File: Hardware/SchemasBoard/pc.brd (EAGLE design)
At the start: 14.9 x 24.1 mm, 10 parts

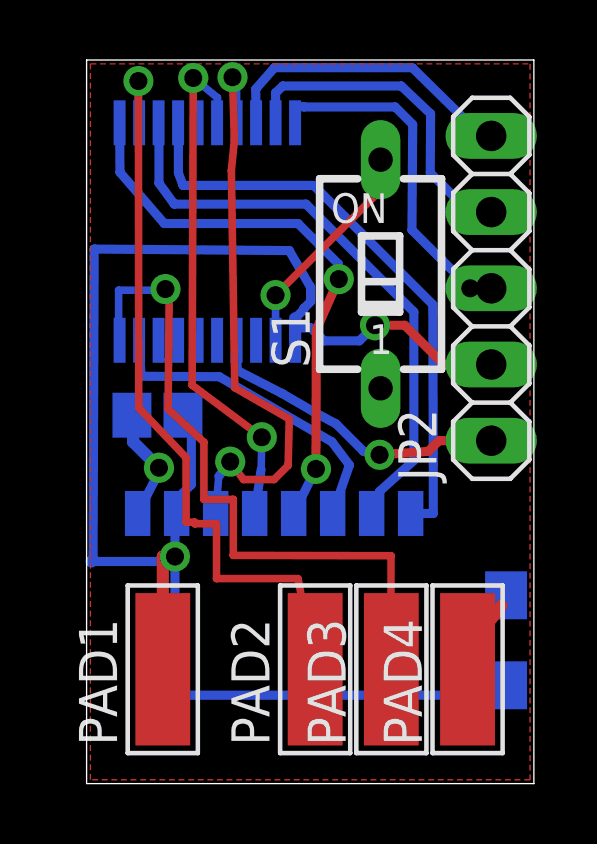
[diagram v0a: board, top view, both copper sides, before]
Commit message: a
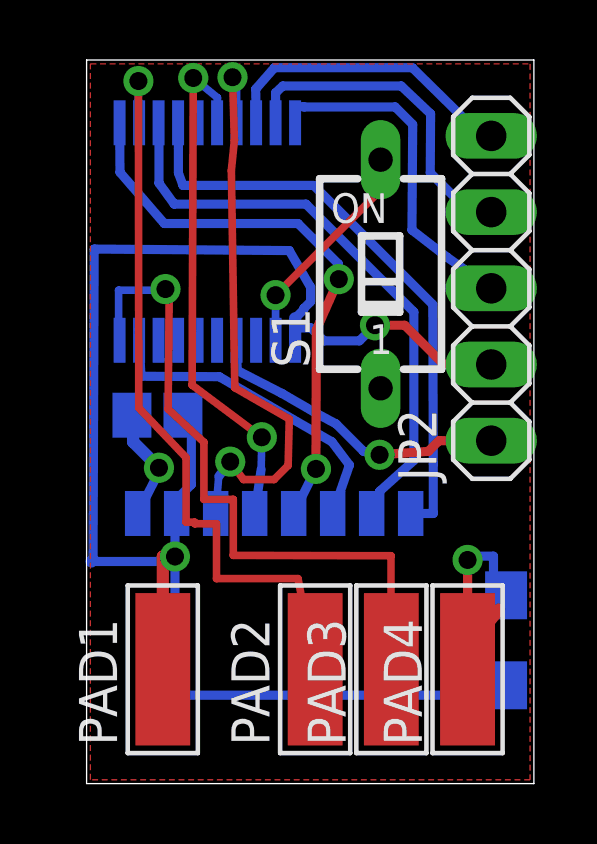
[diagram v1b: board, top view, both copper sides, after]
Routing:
- net GND: track 19.0 -> 23.9 mm
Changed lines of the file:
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@@
 <contactref element="PAD4" pad="1"/>
 <contactref element="S1" pad="1"/>
-<wire x1="13.488290625" y1="16.51" x2="12.7889" y2="16.51" width="0.3048" layer="16"/>
-<wire x1="12.7889" y1="16.51" x2="10.8458" y2="18.4531" width="0.3048" layer="16"/>
 <wire x1="10.8458" y1="18.4531" x2="10.8712" y2="21.971" width="0.3048" layer="16"/>
 <wire x1="10.8712" y1="21.971" x2="10.287" y2="22.5552" width="0.3048" layer="16"/>
@@
 <contactref element="C1" pad="2"/>
 <contactref element="C2" pad="-"/>
-<wire x1="13.8303" y1="5.9436" x2="13.7541" y2="5.8039" width="0.4064" layer="1"/>
-<wire x1="13.7541" y1="5.8039" x2="12.0904" y2="3.8354" width="0.4064" layer="1"/>
+<wire x1="13.7541" y1="5.8039" x2="13.136665625" y2="5.073346875" width="0.4064" layer="1"/>
+<wire x1="13.136665625" y1="5.073346875" x2="12.0904" y2="3.8354" width="0.4064" layer="1"/>
 <wire x1="12.0904" y1="3.8354" x2="12.7" y2="3.8354" width="0.4064" layer="1"/>
 <wire x1="12.7" y1="3.8354" x2="12.7" y2="3.81" width="0.4064" layer="1"/>
@@
 <wire x1="1.5494" y1="11.3919" x2="1.5494" y2="12.2437" width="0.4064" layer="16"/>
 <wire x1="1.5494" y1="12.2437" x2="1.5122" y2="12.2809" width="0.4064" layer="16"/>
-<via x="12.7889" y="16.51" extent="1-16" drill="0.6" shape="square"/>
-<wire x1="13.8303" y1="5.9436" x2="13.9827" y2="6.2752" width="0" layer="19" extent="1-16"/>
+<wire x1="13.9827" y1="6.2752" x2="13.5636" y2="6.2752" width="0.3048" layer="16"/>
+<wire x1="13.5636" y1="6.2752" x2="13.5636" y2="7.5819" width="0.3048" layer="16"/>
+<wire x1="13.5636" y1="7.5819" x2="12.7" y2="7.5819" width="0.3048" layer="16"/>
+<wire x1="12.7" y1="7.5819" x2="12.7" y2="7.4549" width="0.3048" layer="16"/>
+<via x="12.7" y="7.4549" extent="1-16" drill="0.6"/>
+<wire x1="12.7" y1="7.4549" x2="12.7" y2="5.5100125" width="0.3048" layer="1"/>
+<wire x1="12.7" y1="5.5100125" x2="13.136665625" y2="5.073346875" width="0.3048" layer="1"/>
+<wire x1="10.8458" y1="18.4531" x2="12.027790625" y2="17.5387" width="0.3048" layer="16"/>
+<wire x1="12.027790625" y1="17.5387" x2="13.488290625" y2="16.51" width="0.3048" layer="16"/>
 </signal>
 <signal name="N$12">
